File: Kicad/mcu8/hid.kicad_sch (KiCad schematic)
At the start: 29 parts, among them IC301 MICROCHIP-MCP2221A-ISL, K301 FRONT #1, K302 FRONT #2, K303 VIN, K304 +5V, K305 FRONT #3, K306 SERVO LEFT, K307 LEFT, K308 USB/UART, K309 SERVO RIGHT, K310 RIGHT

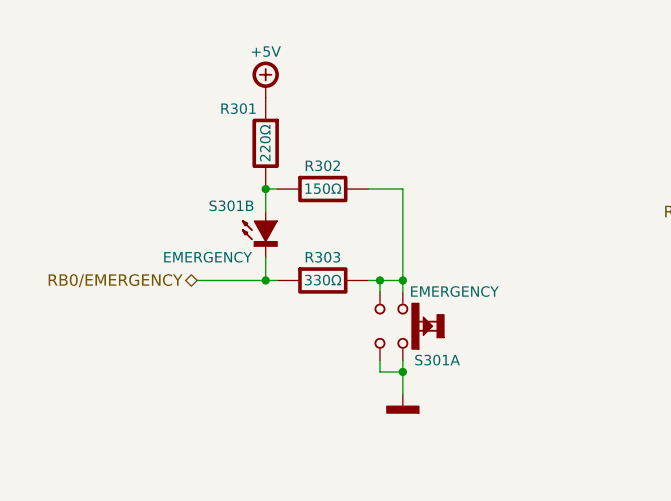
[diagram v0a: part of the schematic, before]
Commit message: Update
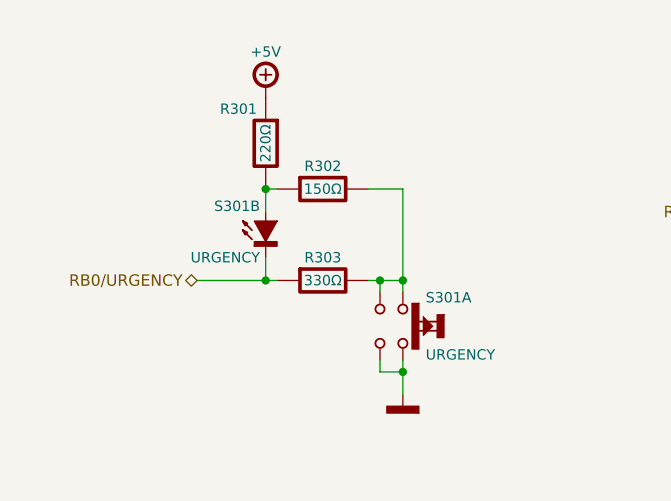
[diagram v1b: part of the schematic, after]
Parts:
- removed S301: EMERGENCY, tronixio:E-SWITCH-TL1240XQ1JXXX, symbol tronixio:E-SWITCH-TL1240RQ1JCLR
- added S301: URGENCY, tronixio:zzzOMRON-B3W9000-X1, symbol tronixio:OMRON-B3W-9000-R1R
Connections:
- net GND: now also S301.3, S301.4
- net at R302.1, R303.1: now also S301.1, S301.2
- net at R301.1, R302.2: now also S301.6 (A)
- net RB0/EMERGENCY renamed RB0/URGENCY
- net RB0/URGENCY: now also S301.5 (C)
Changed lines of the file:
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@@
     (effects (font (size 1.27 1.27)) (justify left))
   )
-  (hierarchical_label "RB0{slash}EMERGENCY" (shape bidirectional) (at 66.04 167.64 180)
+  (hierarchical_label "RB0{slash}URGENCY" (shape bidirectional) (at 66.04 167.64 180)
     (effects (font (size 1.27 1.27)) (justify right))
   )
@@
     )
     (pin "1")
+  )
+  (symbol (lib_id "tronixio:OMRON-B3W-9000-R1R") (at 88.9 172.72 270) (unit 1)
+    (in_bom yes) (on_board yes)
+    (property "Reference" "S301" (id 0) (at 91.44 169.545 90)
+      (effects (font (size 1.15 1.15)) (justify left))
+    )
+    (property "Value" "URGENCY" (id 1) (at 91.44 175.895 90)
+      (effects (font (size 1.15 1.15)) (justify left))
+    )
+    (property "Footprint" "tronixio:zzzOMRON-B3W9000-X1" (id 2) (at 81.28 172.72 0)
+      (effects (font (size 1 1)) hide)
+    )
+    (property "Datasheet" "https://components.omron.com/us-en/datasheet_pdf/A167-E1.pdf" (id 3) (at 78.74 172.72 0)
+      (effects (font (size 1 1)) hide)
+    )
+    (property "Mouser" "653-B3W-9000-R1R" (id 4) (at 76.2 172.72 0)
+      (effects (font (size 1 1)) hide)
+    )
+    (pin "1")
+    (pin "2")
+    (pin "3")
+    (pin "4")
+    (pin "5")
+    (pin "6")
   )
   (symbol (lib_id "tronixio:R-1206") (at 80.01 167.64 270) (unit 1)
@@
     (pin "2")
   )
-  (symbol (lib_id "tronixio:E-SWITCH-TL1240RQ1JCLR") (at 88.9 172.72 270) (mirror x) (unit 1)
-    (in_bom yes) (on_board yes)
-    (property "Reference" "S301" (id 0) (at 92.71 176.53 90)
-      (effects (font (size 1.15 1.15)))
-    )
-    (property "Value" "EMERGENCY" (id 1) (at 94.615 168.91 90)
-      (effects (font (size 1.15 1.15)))
-    )
-    (property "Footprint" "tronixio:E-SWITCH-TL1240XQ1JXXX" (id 2) (at 81.28 172.72 0)
-      (effects (font (size 1 1)) hide)
-    )
-    (property "Datasheet" "https://www.e-switch.com/product-catalog/tact/product-lines/tl1240-series-illuminated-tact-switches#.XnJ2Ri2ZPUI" (id 3) (at 78.74 172.72 0)
-      (effects (font (size 1 1)) hide)
-    )
-    (property "Mouser" "612-TL1240RQ1JCLR" (id 4) (at 76.2 172.72 0)
-      (effects (font (size 1 1)) hide)
-    )
-    (pin "1")
-    (pin "2")
-    (pin "3")
-    (pin "4")
-    (pin "5")
-    (pin "6")
-  )
   (symbol (lib_id "tronixio:POWER-+5V") (at 134.62 101.6 0) (mirror y) (unit 1)
     (in_bom yes) (on_board yes)
@@
     (pin "2")
   )
+  (symbol (lib_id "tronixio:OMRON-B3W-9000-R1R") (at 73.66 162.56 90) (unit 2)
+    (in_bom yes) (on_board yes)
+    (property "Reference" "S301" (id 0) (at 73.025 159.385 90)
+      (effects (font (size 1.15 1.15)) (justify left))
+    )
+    (property "Value" "URGENCY" (id 1) (at 73.025 165.1 90)
+      (effects (font (size 1.15 1.15)) (justify left))
+    )
+    (property "Footprint" "tronixio:zzzOMRON-B3W9000-X1" (id 2) (at 81.28 162.56 0)
+      (effects (font (size 1 1)) hide)
+    )
+    (property "Datasheet" "https://components.omron.com/us-en/datasheet_pdf/A167-E1.pdf" (id 3) (at 83.82 162.56 0)
+      (effects (font (size 1 1)) hide)
+    )
+    (property "Mouser" "653-B3W-9000-R1R" (id 4) (at 86.36 162.56 0)
+      (effects (font (size 1 1)) hide)
+    )
+    (pin "1")
+    (pin "2")
+    (pin "3")
+    (pin "4")
+    (pin "5")
+    (pin "6")
+  )
   (symbol (lib_id "tronixio:R-1206") (at 80.01 157.48 270) (unit 1)
     (in_bom yes) (on_board yes)
@@
     (pin "5")
   )
-  (symbol (lib_id "tronixio:E-SWITCH-TL1240RQ1JCLR") (at 73.66 162.56 90) (unit 2)
-    (in_bom yes) (on_board yes)
-    (property "Reference" "S301" (id 0) (at 67.31 159.385 90)
-      (effects (font (size 1.15 1.15)) (justify right))
-    )
-    (property "Value" "EMERGENCY" (id 1) (at 62.23 165.1 90)
-      (effects (font (size 1.15 1.15)) (justify right))
-    )
-    (property "Footprint" "tronixio:E-SWITCH-TL1240XQ1JXXX" (id 2) (at 81.28 162.56 0)
-      (effects (font (size 1 1)) hide)
-    )
-    (property "Datasheet" "https://www.e-switch.com/product-catalog/tact/product-lines/tl1240-series-illuminated-tact-switches#.XnJ2Ri2ZPUI" (id 3) (at 83.82 162.56 0)
-      (effects (font (size 1 1)) hide)
-    )
-    (property "Mouser" "612-TL1240RQ1JCLR" (id 4) (at 86.36 162.56 0)
-      (effects (font (size 1 1)) hide)
-    )
-    (pin "1")
-    (pin "2")
-    (pin "3")
-    (pin "4")
-    (pin "5")
-    (pin "6")
-  )
   (symbol (lib_id "tronixio:C-1206") (at 200.66 73.66 0) (unit 1)

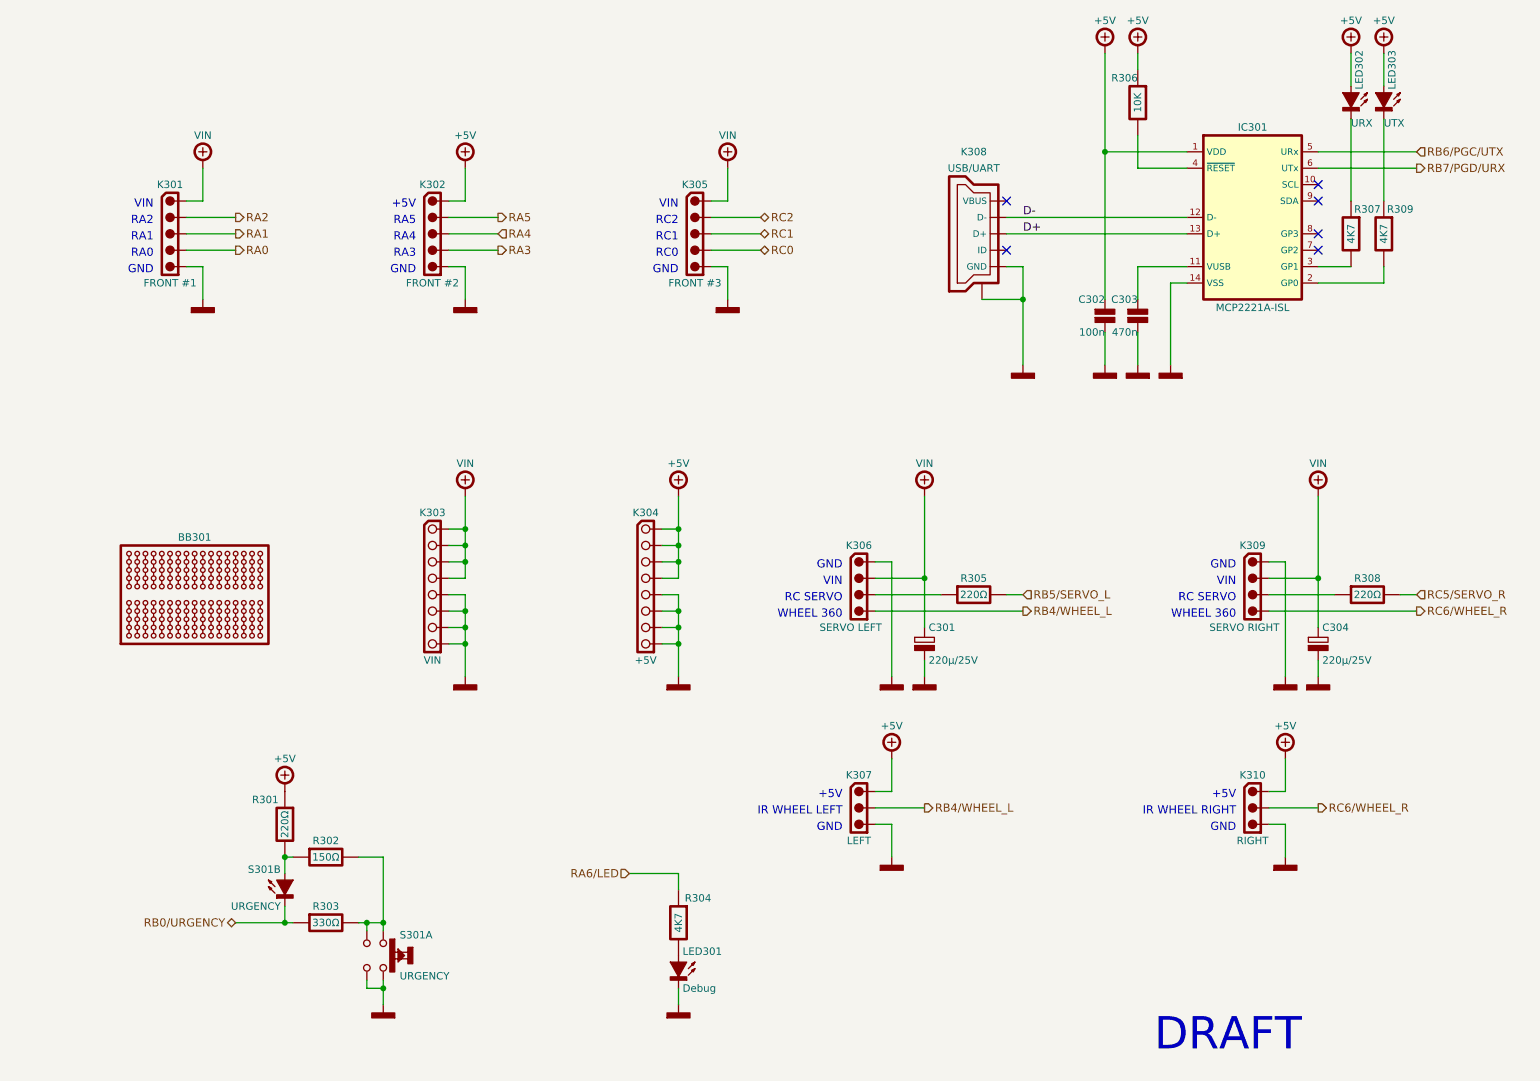
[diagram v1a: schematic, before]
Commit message: Update
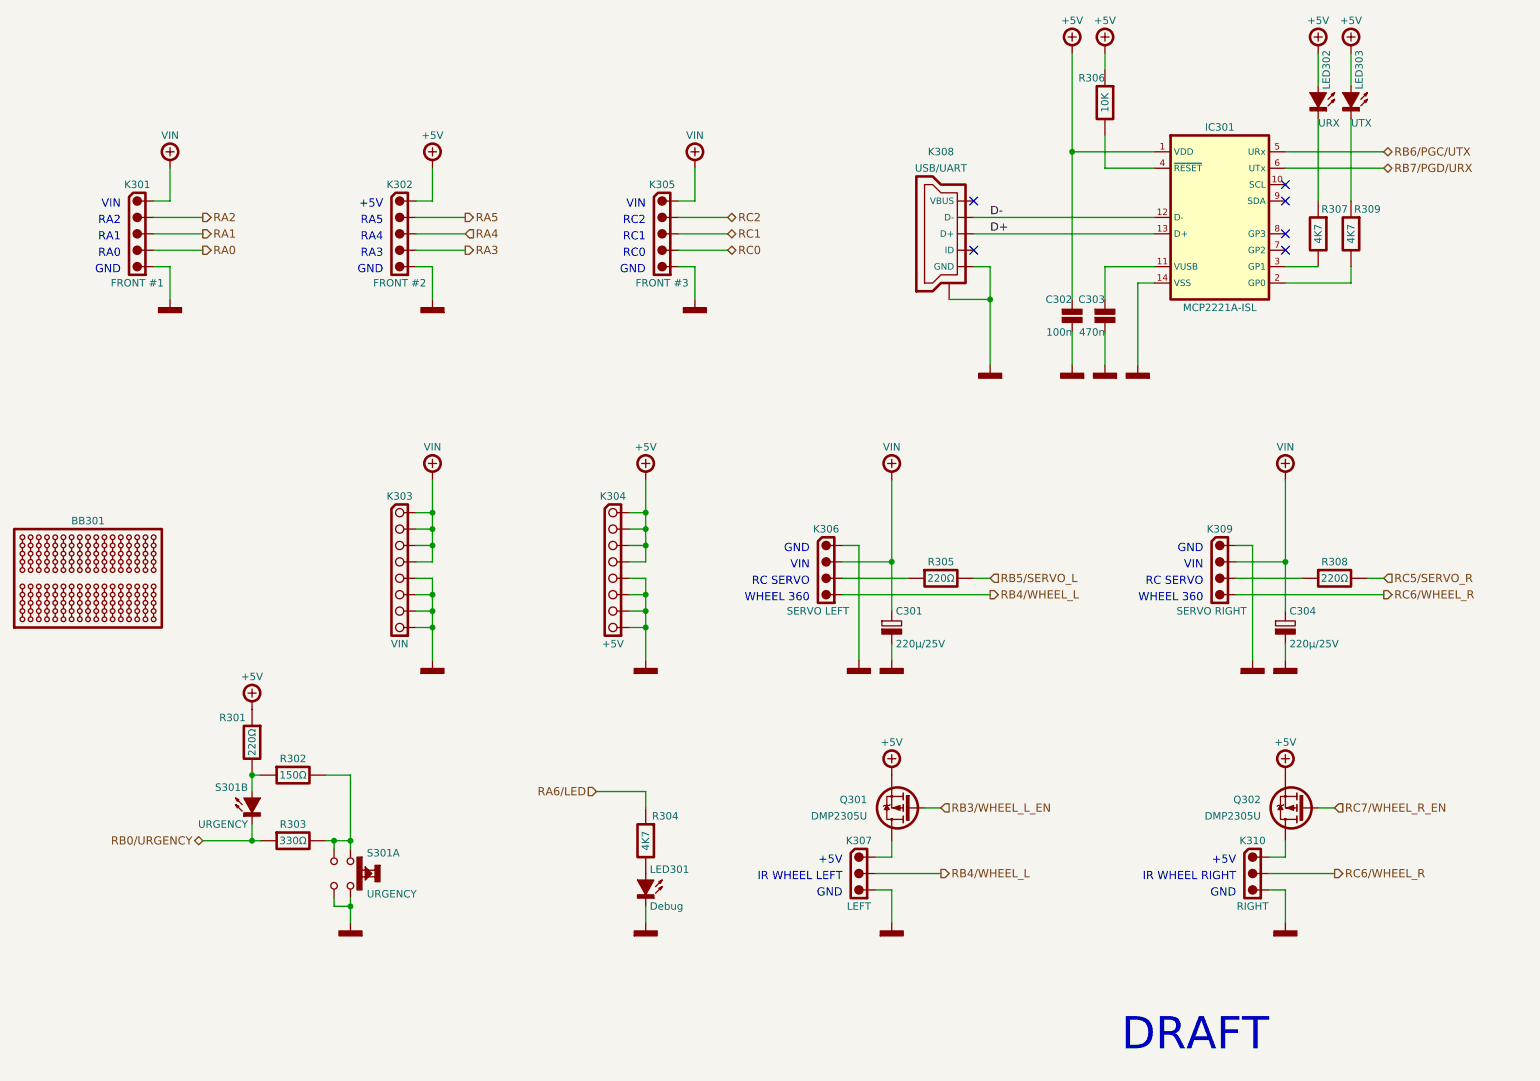
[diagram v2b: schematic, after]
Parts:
- added Q301, Q302: DIODESINC-DMP2305U-SOT-23, tronixio:SOT-23-3, symbol tronixio:DIODESINC-DMP2305U-SOT-23
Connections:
- net +5V: now also Q301.2 (S), Q302.2 (S); no longer K307.1, K310.1
- new net: K310.1, Q302.3 (D)
- new net: K307.1, Q301.3 (D)
- new net RB3/WHEEL_L_EN: Q301.1 (G)
- new net RC7/WHEEL_R_EN: Q302.1 (G)
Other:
- moved on the sheet: BB301, C301, C302, C303, C304, IC301, K301, K302, K303, K304, K305, K306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

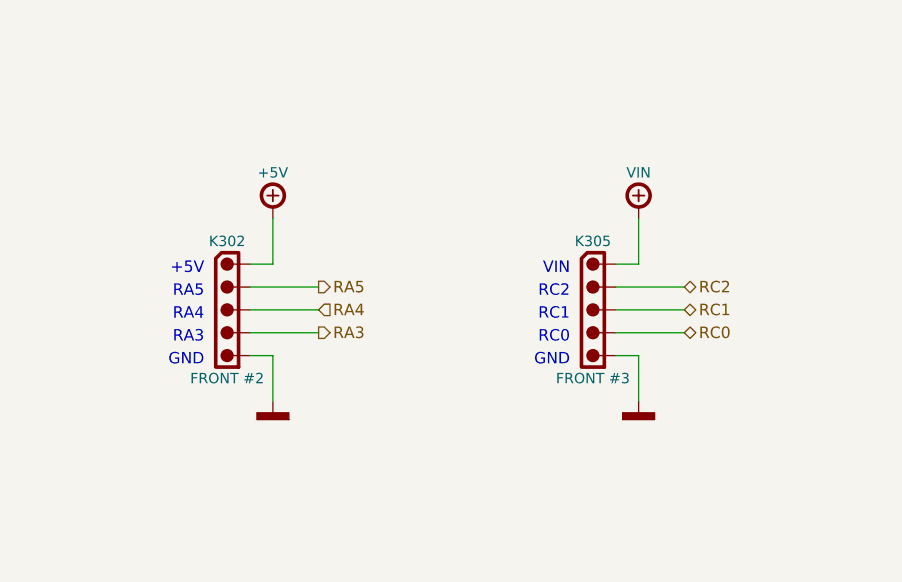
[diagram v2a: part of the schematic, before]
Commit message: Update
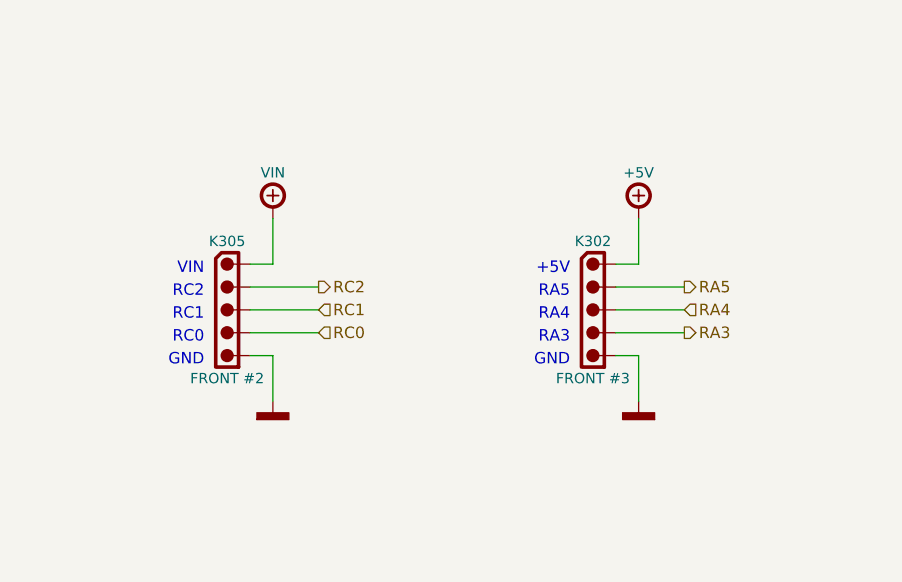
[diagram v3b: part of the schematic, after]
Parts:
- K302: value FRONT #2 -> FRONT #3
- K305: value FRONT #3 -> FRONT #2
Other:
- moved on the sheet: K302, K305
